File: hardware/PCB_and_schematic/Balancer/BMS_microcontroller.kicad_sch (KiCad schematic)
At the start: 43 parts, among them J10 RS485, J8 ICP, J9 Conn_01x03, Q17 BC817, Q18 BC817, Q19 BC817, Q20 BC817, U4 PIC16F886-IP, U5 TL431LP, U6 ST485, U7 INA226

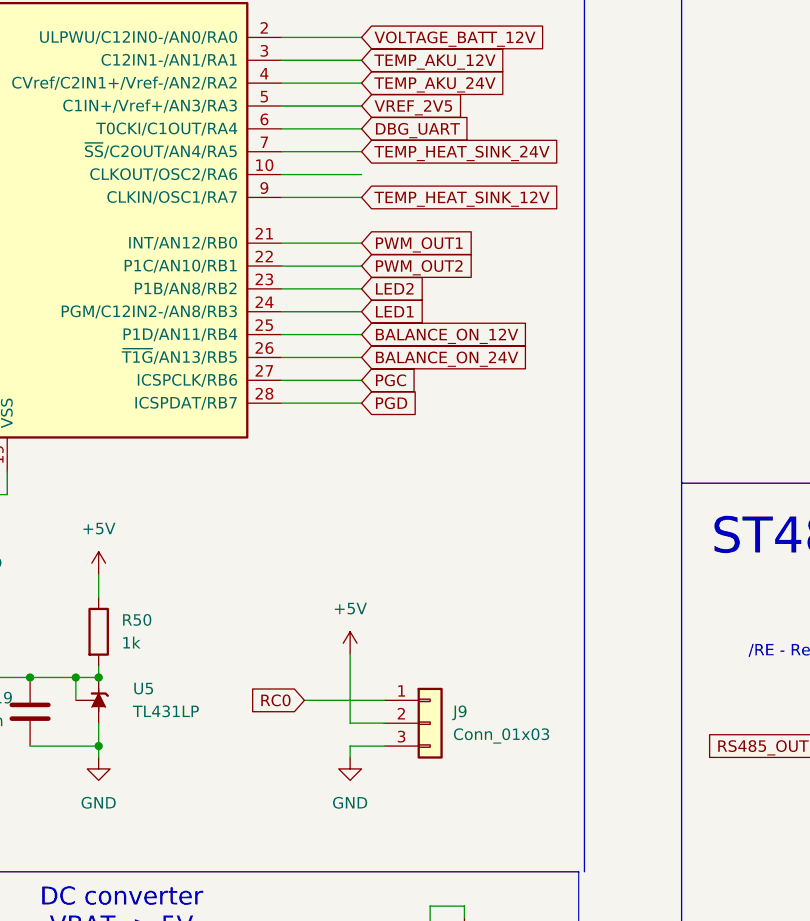
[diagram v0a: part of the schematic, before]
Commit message: Route balancer progress
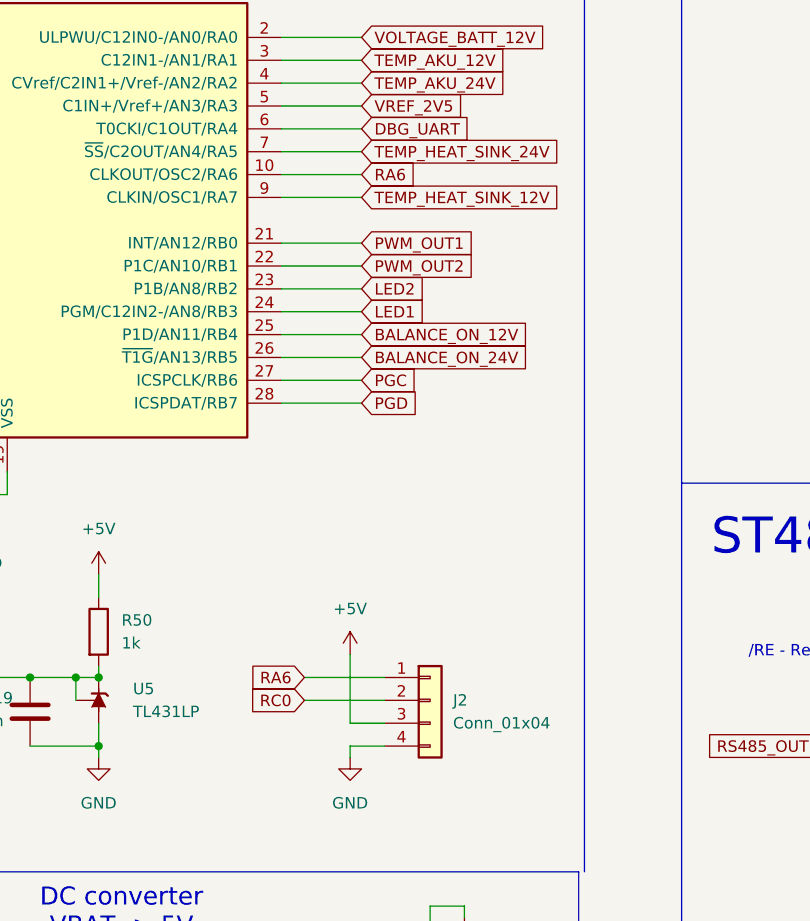
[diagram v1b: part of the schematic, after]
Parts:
- removed J9: Conn_01x03, Connector_PinHeader_2.54mm:PinHeader_1x03_P2.54mm_Vertical, symbol Connector_Generic:Conn_01x03
- added J2: Conn_01x04, Connector_PinHeader_2.54mm:PinHeader_1x04_P2.54mm_Vertical, symbol Connector_Generic:Conn_01x04
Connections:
- net +5V: now also J2.3 (Pin_3)
- net GND: now also J2.4 (Pin_4)
- net RC0: now also J2.2 (Pin_2)
- net RA6: now reaches U4.10 (CLKOUT/OSC2/RA6)
- net RA6: now also J2.1 (Pin_1)
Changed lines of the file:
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@@
 	(wire
 		(pts
+			(xy 129.54 123.19) (xy 138.43 123.19)
+		)
+		(stroke
+			(width 0)
+			(type default)
+		)
+	)
+	(wire
+		(pts
 			(xy 234.95 135.89) (xy 234.95 139.7)
 		)
@@
 		)
 	)
+	(global_label "RA6"
+		(shape input)
+		(at 129.54 123.19 180)
+		(fields_autoplaced yes)
+		(effects
+			(font
+				(size 1.27 1.27)
+			)
+			(justify right)
+		)
+		(property "Intersheetrefs" "${INTERSHEET_REFS}"
+			(at 122.9867 123.19 0)
+			(effects
+				(font
+					(size 1.27 1.27)
+				)
+				(justify right)
+				(hide yes)
+			)
+		)
+	)
 	(global_label "RS232_TX"
 		(shape input)
@@
 		)
 	)
+	(global_label "RA6"
+		(shape input)
+		(at 135.89 67.31 0)
+		(fields_autoplaced yes)
+		(effects
+			(font
+				(size 1.27 1.27)
+			)
+			(justify left)
+		)
+		(property "Intersheetrefs" "${INTERSHEET_REFS}"
+			(at 142.4433 67.31 0)
+			(effects
+				(font
+					(size 1.27 1.27)
+				)
+				(justify left)
+				(hide yes)
+			)
+		)
+	)
 	(global_label "VREF_2V5"
 		(shape input)
@@
 	)
 	(symbol
+		(lib_id "Connector_Generic:Conn_01x04")
+		(at 143.51 125.73 0)
+		(unit 1)
+		(exclude_from_sim no)
+		(in_bom yes)
+		(on_board yes)
+		(dnp no)
+		(fields_autoplaced yes)
+		(property "Reference" "J2"
+			(at 146.05 125.7299 0)
+			(effects
+				(font
+					(size 1.27 1.27)
+				)
+				(justify left)
+			)
+		)
+		(property "Value" "Conn_01x04"
+			(at 146.05 128.2699 0)
+			(effects
+				(font
+					(size 1.27 1.27)
+				)
+				(justify left)
+			)
+		)
+		(property "Footprint" "Connector_PinHeader_2.54mm:PinHeader_1x04_P2.54mm_Vertical"
+			(at 143.51 125.73 0)
+			(effects
+				(font
+					(size 1.27 1.27)
+				)
+				(hide yes)
+			)
+		)
+		(property "Datasheet" "~"
+			(at 143.51 125.73 0)
+			(effects
+				(font
+					(size 1.27 1.27)
+				)
+				(hide yes)
+			)
+		)
+		(property "Description" "Generic connector, single row, 01x04, script generated (kicad-library-utils/schlib/autogen/connector/)"
+			(at 143.51 125.73 0)
+			(effects
+				(font
+					(size 1.27 1.27)
+				)
+				(hide yes)
+			)
+		)
+		(pin "3"
+		)
+		(pin "2"
+		)
+		(pin "4"
+		)
+		(pin "1"
+		)
+		(instances
+			(project "Balancer"
+				(path "/555ba40f-9abb-4b99-82c6-07e888fda9fd/3b90ff07-e5cb-404b-939d-de320e975ba1"
+					(reference "J2")
+					(unit 1)
+				)
+			)
+		)
+	)
+	(symbol
 		(lib_id "power:+5V")
 		(at 156.21 158.75 0)
@@
 					(unit 1)
 				)
-			)
-		)
-	)
-	(symbol
-		(lib_id "Connector_Generic:Conn_01x03")
-		(at 143.51 128.27 0)
-		(unit 1)
-		(exclude_from_sim no)
-		(in_bom yes)
-		(on_board yes)
-		(dnp no)
-		(fields_autoplaced yes)
-		(property "Reference" "J9"
-			(at 146.05 126.9999 0)
-			(effects
-				(font
-					(size 1.27 1.27)
-				)
-				(justify left)
-			)
-		)
-		(property "Value" "Conn_01x03"
-			(at 146.05 129.5399 0)
-			(effects
-				(font
-					(size 1.27 1.27)
-				)
-				(justify left)
-			)
-		)
-		(property "Footprint" "Connector_PinHeader_2.54mm:PinHeader_1x03_P2.54mm_Vertical"
-			(at 143.51 128.27 0)
-			(effects
-				(font
-					(size 1.27 1.27)
-				)
-				(hide yes)
-			)
-		)
-		(property "Datasheet" "~"
-			(at 143.51 128.27 0)
-			(effects
-				(font
-					(size 1.27 1.27)
-				)
-				(hide yes)
-			)
-		)
-		(property "Description" "Generic connector, single row, 01x03, script generated (kicad-library-utils/schlib/autogen/connector/)"
-			(at 143.51 128.27 0)
-			(effects
-				(font
-					(size 1.27 1.27)
-				)
-				(hide yes)
-			)
-		)
-		(pin "3"
-		)
-		(pin "1"
-		)
-		(pin "2"
-		)
-		(instances
-			(project "Balancer"
-				(path "/555ba40f-9abb-4b99-82c6-07e888fda9fd/3b90ff07-e5cb-404b-939d-de320e975ba1"
-					(reference "J9")
-					(unit 1)
-				)
